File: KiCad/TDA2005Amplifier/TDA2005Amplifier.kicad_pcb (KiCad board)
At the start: 2 copper layers, 74.9 x 76.8 mm, 30 parts, among them J1 Audio In, U1 Vol R, U2 Vol L, U3 TDA2005, U4 Speakers, U5 Power In

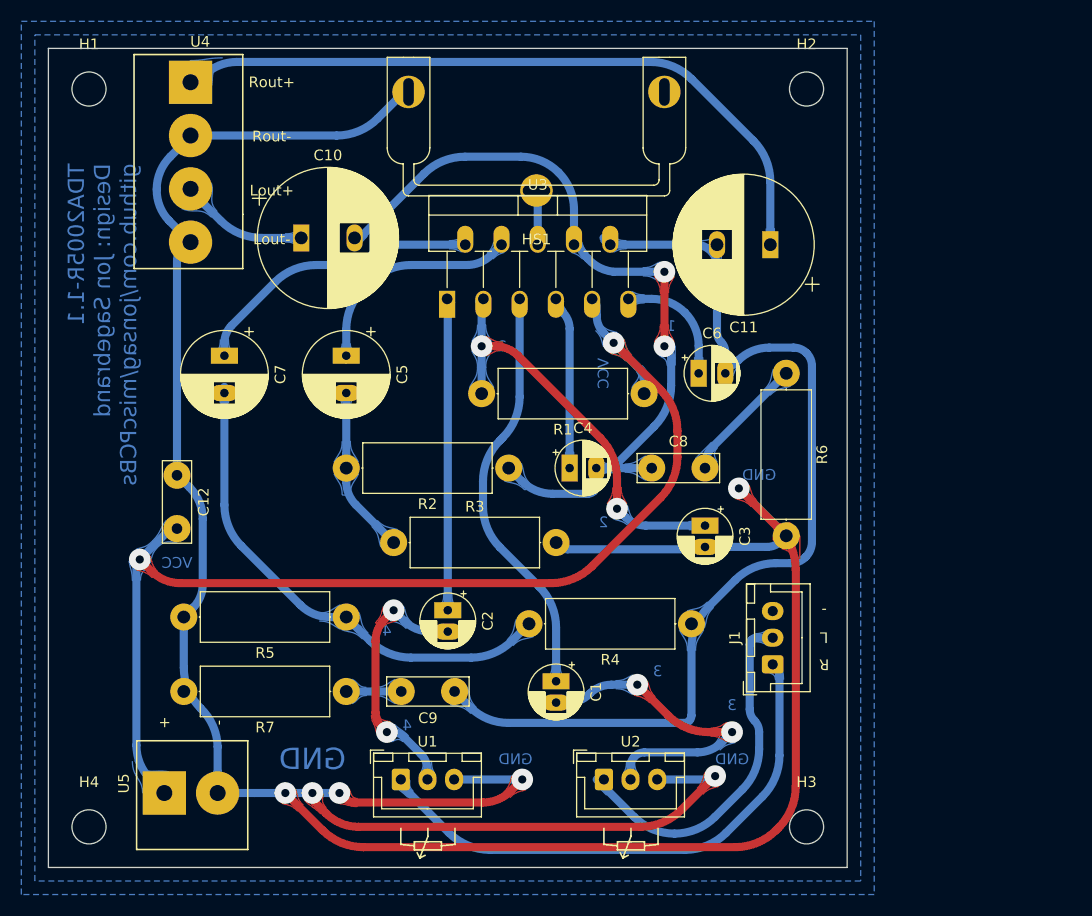
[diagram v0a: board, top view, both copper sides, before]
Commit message: PCBs
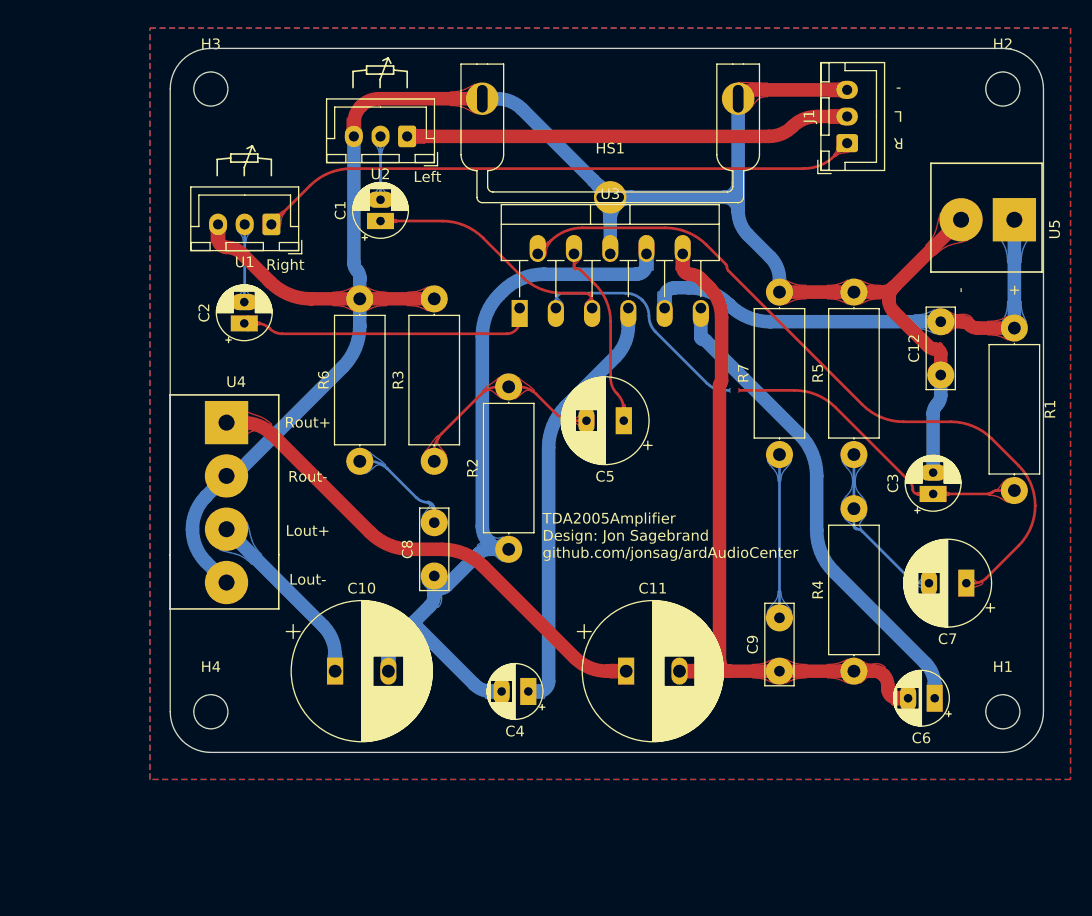
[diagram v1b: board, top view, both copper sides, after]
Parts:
- moved H1 103.7 mm to (238.4, -54.5)
- moved U5 96.2 mm to (239.4, -100.7), turned to -90 degrees
- moved H3 89.0 mm to (164.1, -112.9)
- moved C7 72.8 mm to (234.9, -66.6), turned to 180 degrees
- moved C12 72.3 mm to (232.5, -86.1), turned to 90 degrees
- moved U2 63.1 mm to (182.5, -108.5), turned to 180 degrees
- moved U1 53.5 mm to (169.8, -100.2), turned to 180 degrees
- moved R5 50.0 mm to (224.4, -78.7), turned to 90 degrees
- moved J1 49.4 mm to (223.8, -107.9)
- moved R7 46.3 mm to (217.4, -78.7), turned to 90 degrees
- moved C1 46.2 mm to (180.0, -100.6), turned to 90 degrees
- moved C11 42.2 mm to (203.0, -58.3), turned to 0 degrees
- moved R6 40.8 mm to (178.0, -78.0), turned to 90 degrees
- moved C10 40.8 mm to (175.7, -58.3)
- moved C6 37.7 mm to (232.0, -55.8), turned to 180 degrees
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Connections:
- net Net-(C10-Pad2) renamed /OpOutL
- net Net-(C11-Pad2) renamed /OpOutR
- net Net-(C4-Pad1) renamed /Op7
- net Net-(C6-Pad1) renamed /Op11
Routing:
- net GND: track 288.2 -> 199.1 mm, vias 6 -> 0
- net +15V: track 106.6 -> 45.4 mm, vias 2 -> 0
- net Net-(C7-Pad1): track 27.8 -> 69.1 mm
- net /Op11: track 11.4 -> 45.1 mm
- net Net-(C7-Pad2): track 47.1 -> 15.9 mm
- net /OpOutR: track 93.7 -> 65.8 mm
- net Net-(C1-Pad2): track 30.6 -> 5.94 mm, vias 2 -> 0
- net /Op7: track 15.7 -> 40.1 mm
- net Rout: track 66.6 -> 46.2 mm
- net Net-(C2-Pad2): track 24.6 -> 7.30 mm, vias 2 -> 0
- net Net-(C1-Pad1): track 38.8 -> 23.2 mm
- net Net-(C3-Pad1): track 39.3 -> 52.5 mm, vias 2 -> 1
- net Net-(C9-Pad2): track 5.80 -> 15.3 mm
- net Lin: track 33.7 -> 41.7 mm
- net Rin: track 51.5 -> 56.7 mm
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- added copper zone on F.Cu, net GND
- removed copper zone on B.Cu, net (none)
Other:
- board size 74.9 x 76.8 mm -> 81.9 x 66 mm
- rule pad_to_mask_clearance: 0.051 -> 0
- board text added: "58,420mm"
- board text added: "74,295mm"
- board text added: "Left"
- board text added: "Right"
- board text added: "TDA2005Amplifier Design: Jon Sagebrand github.com/jonsag/ardAudioCenter"
- board text removed: "1"
- board text removed: "2"
- board text removed: "3"
- board text removed: "4"
- board text removed: "GND"
- board text removed: "TDA2005R-1.1 Design: Jon Sagebrand github.com/jonsag/miscPCBs"
- board text removed: "VCC"
